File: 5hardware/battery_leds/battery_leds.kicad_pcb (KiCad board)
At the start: 2 copper layers, 32 x 32 mm, 31 parts, among them J1 Conn_01x03_Pin, Q1 AO3400A, Q2 AO3400A, SW2 SW_Push

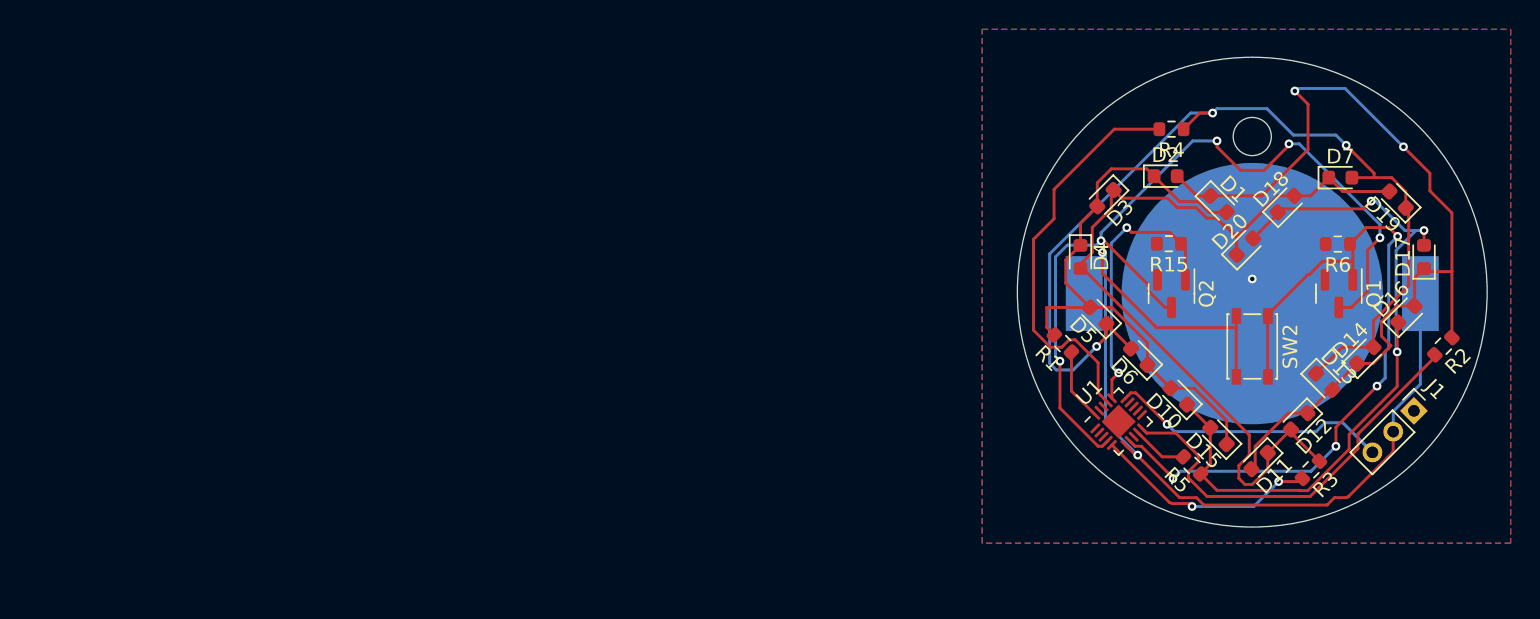
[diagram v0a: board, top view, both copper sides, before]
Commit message: udpate PCBs.
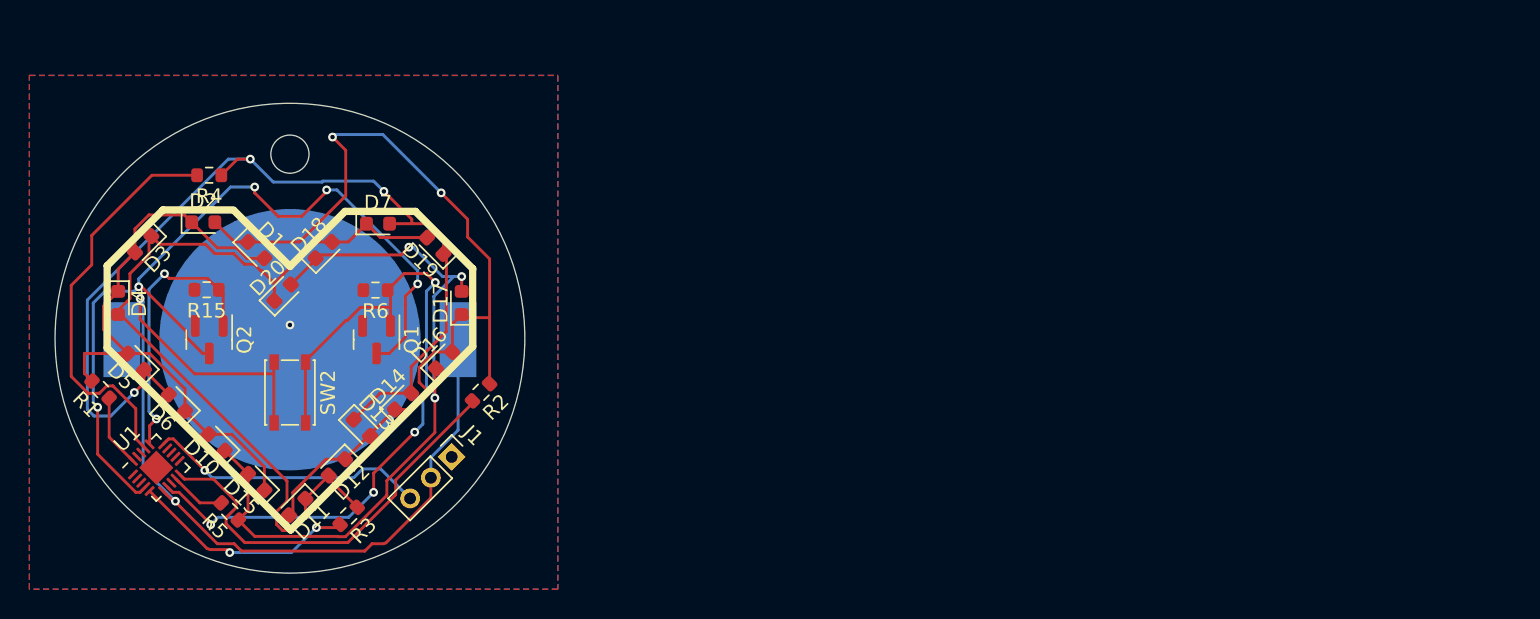
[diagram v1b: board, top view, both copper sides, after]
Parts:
- moved BT2 65.6 mm to (147.5, 96.4)
- moved D10 65.6 mm to (142.5, 103.4)
- moved D11 65.6 mm to (148.0, 107.8)
- moved D13 65.6 mm to (152.4, 102.4)
- moved D16 65.6 mm to (158.0, 97.8)
- moved D18 65.6 mm to (149.8, 90.3)
- moved D19 65.6 mm to (157.4, 90.0)
- moved D20 65.6 mm to (147.0, 93.2)
- moved D3 65.6 mm to (137.5, 89.9)
- moved D4 65.6 mm to (135.8, 93.9)
- moved D5 65.6 mm to (137.0, 97.9)
- moved D6 65.6 mm to (139.8, 100.7)
- moved D7 65.6 mm to (153.5, 88.5)
- moved J1 65.6 mm to (158.5, 104.4)
- moved Q1 65.6 mm to (153.4, 96.4)
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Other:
- outline, holes or cut-outs redrawn
- board text added: "3.3V"
- board text added: "GND"
- board text added: "Love & Light Badge_V1.0"
- board text added: "SWIO"
